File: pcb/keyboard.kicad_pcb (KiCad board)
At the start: 2 copper layers, 232.6 x 118.3 mm, 123 parts, among them SW1 Push, SW10 Push, SW11 Push, SW12 Push, SW14 Push, SW15 Push, SW16 Push, SW17 Push, SW18 Push, SW2 Push, SW20 Push, SW21 Push, SW22 Push, SW23 Push, SW24 Push, SW26 Push, SW27 Push, SW28 Push, SW29 Push, SW3 Push, SW30 Push, SW32 Push, SW33 Push, SW34 Push, SW35 Push, SW38 Push, SW39 Push, SW4 Push, SW40 Push, SW41 Push, SW42 Push, SW44 Push, SW45 Push, SW46 Push, SW47 Push, SW48 Push, SW5 Push, SW50 Push, SW51 Push, SW52 Push, SW53 Push, SW54 Push, SW56 Push, SW57 Push, SW58 Push, SW59 Push, SW6 Push, SW60 Push, SW62 Push, SW63 Push, SW64 Push, SW65 Push, SW66 Push, SW67 Push, SW68 Push, SW69 Push, SW70 Push, SW71 Push, SW72 Push, SW8 Push, SW9 Push, U1 Arduino_Pro_Micro

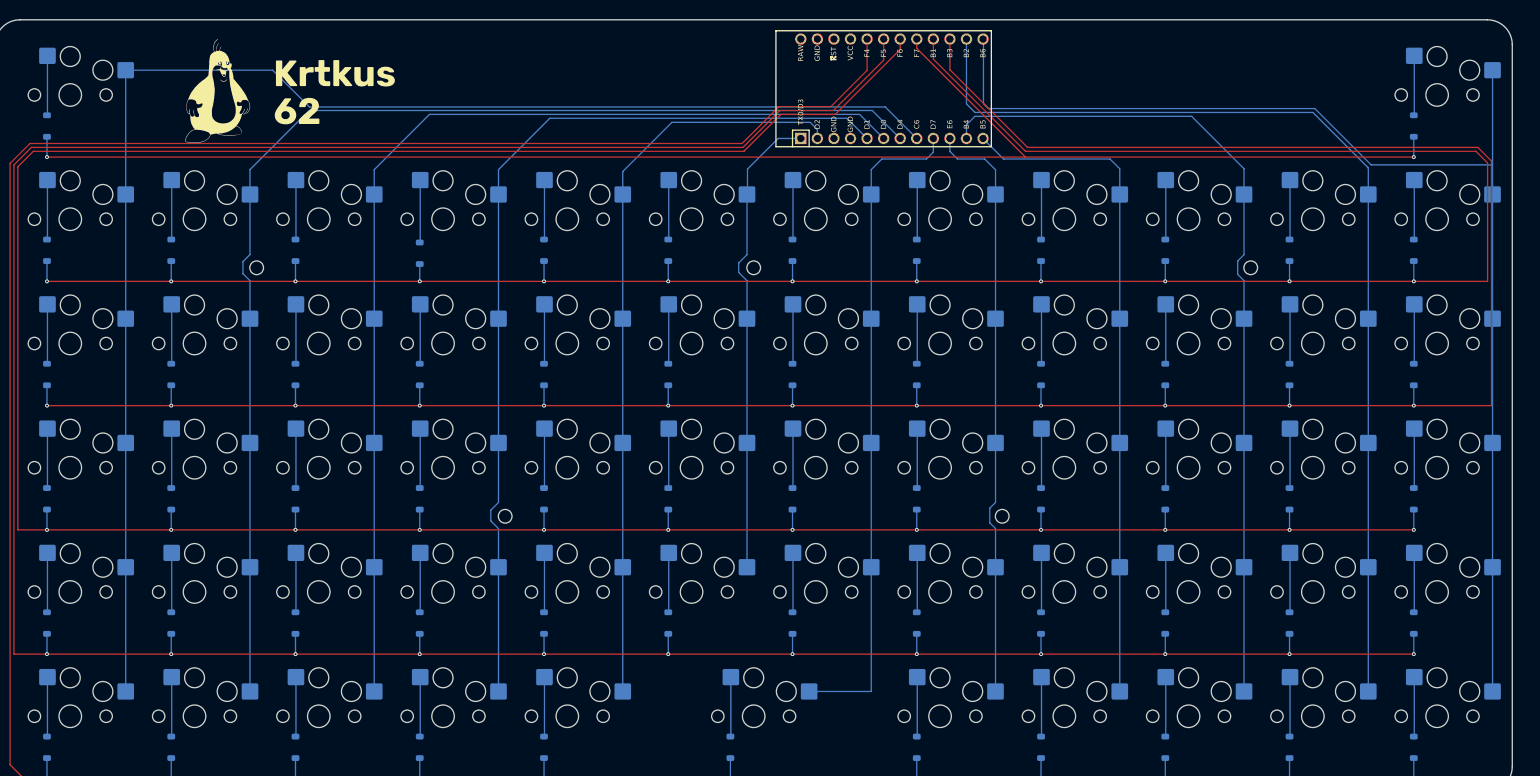
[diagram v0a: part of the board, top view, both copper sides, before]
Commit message: through hole
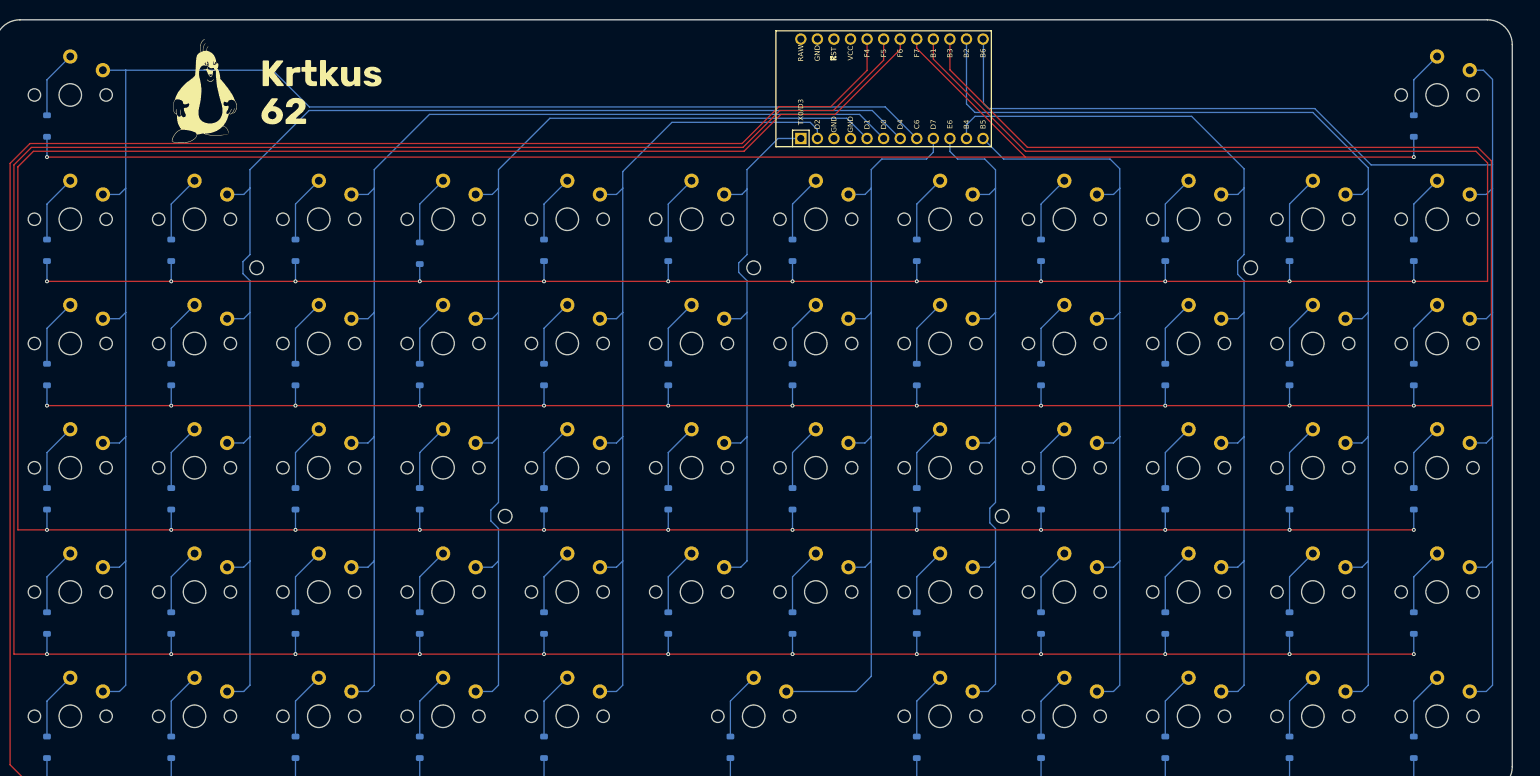
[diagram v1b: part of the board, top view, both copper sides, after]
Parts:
- SW1, SW10, SW11, SW12, SW14, SW15, SW16, SW17, SW18, SW2, SW20, SW21, SW22, SW23, SW24, SW26, SW27, SW28, SW29, SW3, SW30, SW32, SW33, SW34, SW35, SW38, SW39, SW4, SW40, SW41, SW42, SW44, SW45, SW46, SW47, SW48, SW5, SW50, SW51, SW52, SW53, SW54, SW56, SW57, SW58, SW59, SW6, SW60, SW62, SW63, SW64, SW65, SW66, SW67, SW68, SW69, SW70, SW71, SW72, SW8, SW9: footprint ScottoKeebs_Hotswap:Hotswap_Choc_V1_1.00u_No_Silkscreen -> ScottoKeebs_Choc:Choc_V1_1.00u_No_Label
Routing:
- net COL0: track 220.9 -> 242.9 mm
- net COL11: track 187.7 -> 208.9 mm
- net COL8: track 103.0 -> 121.6 mm
- net COL3: track 142.0 -> 160.6 mm
- net COL2: track 163.1 -> 181.7 mm
- net COL1: track 186.1 -> 204.6 mm
- net COL4: track 114.5 -> 133.0 mm
- net COL9: track 129.5 -> 148.0 mm
- net COL10: track 156.6 -> 175.1 mm
- net COL7: track 90.8 -> 109.3 mm
- net COL6: track 102.3 -> 120.0 mm
- net COL5: track 72.2 -> 86.8 mm
- net Net-(D8-A): track 9.14 -> 10.5 mm
- net Net-(D71-A): track 9.14 -> 10.5 mm
- net Net-(D70-A): track 9.14 -> 10.5 mm
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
